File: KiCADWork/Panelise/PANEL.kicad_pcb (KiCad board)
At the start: 2 copper layers, 88.5 x 60.5 mm, 196 parts, among them J1 Screw_Terminal_01x01, J1 Screw_Terminal_01x02, J1 USB_C_Receptacle, J2 Screw_Terminal_01x01, J2 Screw_Terminal_01x02, J3 USB_C_Receptacle, J4 Conn_01x10_Socket, P1 USB_C_Plug, P2 USB_C_Plug, SW1 TK-6580B-1, SW2 SW_DIP_x01, U1 MCP73831T-2ACI/OT, U1 USB2422T-I/MJ, U2 TPS61023DRLR, U2 XB6096I2SV, U3 AMS1117-3.3, U3 NRF52833-QDAA-R7, U4 BQ24073RGT, U5 SIP32509DT-T1-GE3, U6 SIP32509DT-T1-GE3, Y1 X322524MOB4SI, Y1 XL7EL89CKI-111YLC-32M, Y2 X161032768KLD2SI

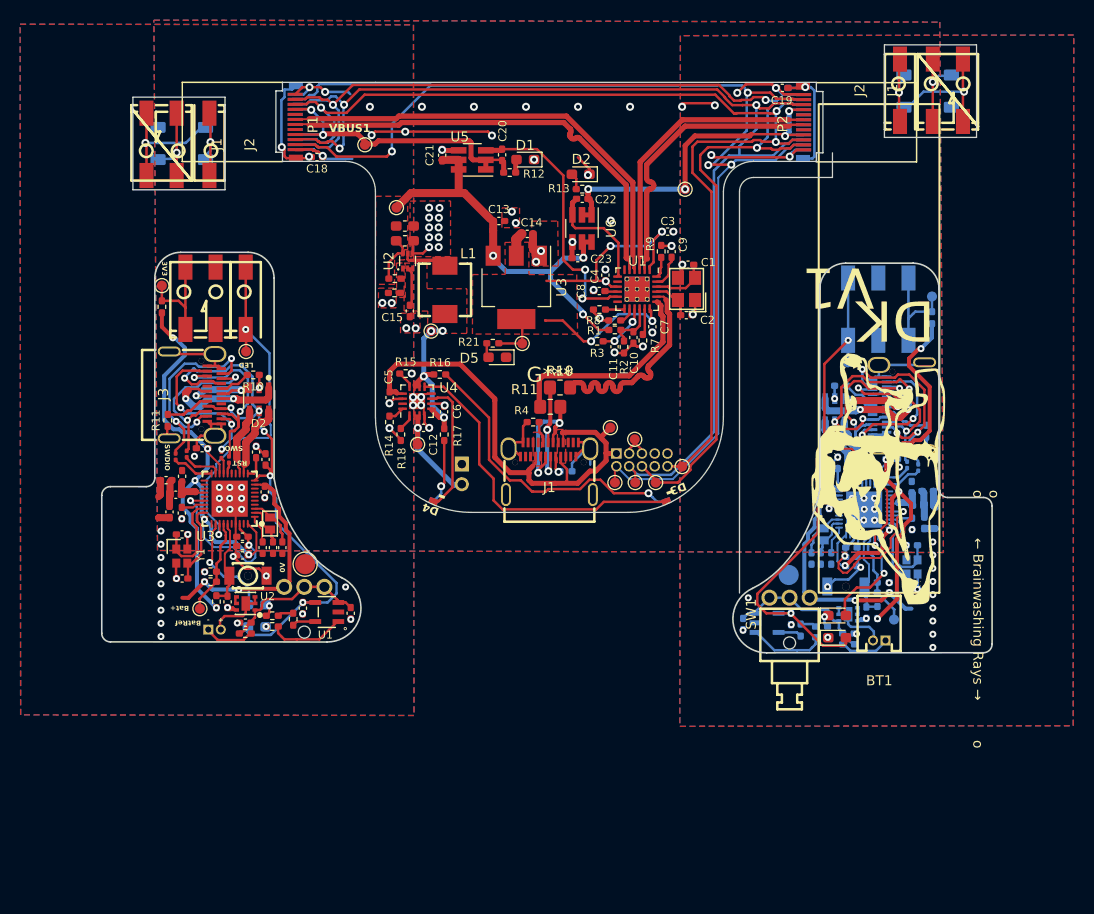
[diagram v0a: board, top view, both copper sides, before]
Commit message: Started mirror earrings and case
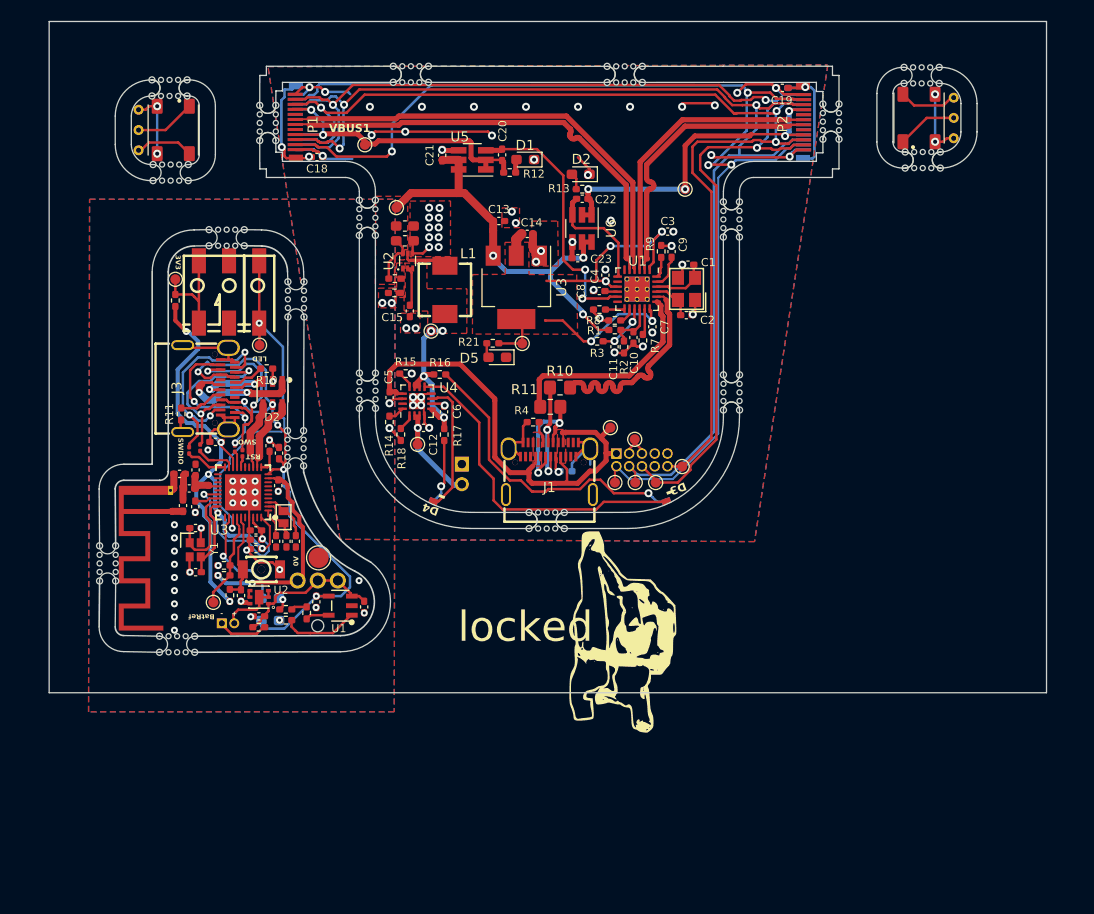
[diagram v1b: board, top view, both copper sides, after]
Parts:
- removed A, B, C, D, E: Board, kikit:Board
- removed the BT1 at (178.3, 114.7)
- removed the BT1 at (112.2, 113.6)
- removed the C1 at (115.0, 106.2)
- removed the C1 at (175.6, 107.3)
- removed the C10 at (117.3, 96.7)
- removed the C10 at (173.3, 97.8)
- removed the C11 at (109.0, 102.0)
- removed the C11 at (181.6, 103.1)
- removed the C12 at (117.2, 99.9)
- removed the C12 at (173.3, 101.0)
- removed the C13 at (125.8, 112.0)
- removed the C13 at (164.8, 113.1)
- removed the C14 at (113.5, 110.9)
- removed the C14 at (177.0, 111.9)
- removed the C15 at (119.0, 105.5)
- removed the C15 at (171.6, 106.6)
- removed the C16 at (118.0, 105.5)
- removed the C16 at (172.5, 106.6)
- removed the C17 at (115.0, 105.3)
- removed the C17 at (175.6, 106.4)
- removed the C18 at (115.3, 112.9)
- removed the C18 at (175.3, 114.0)
- removed the C19 at (121.0, 111.5)
- removed the C19 at (169.6, 112.6)
- removed the C2 at (117.0, 105.5)
- removed the C2 at (173.6, 106.6)
- removed the C3 at (109.0, 104.2)
- removed the C3 at (181.6, 105.2)
- removed the C4 at (109.0, 108.5)
- removed the C4 at (181.6, 109.6)
- removed the C5 at (107.4, 98.8)
- removed the C5 at (183.2, 99.8)
- removed the C6 at (111.0, 95.6)
- removed the C6 at (179.6, 96.7)
- removed the C7 at (115.0, 104.4)
- removed the C7 at (175.6, 105.5)
- removed the C8 at (109.0, 98.4)
- removed the C8 at (181.6, 99.5)
- removed the C9 at (116.4, 96.0)
- removed the C9 at (174.2, 97.0)
- removed the D1 at (174.1, 114.4)
- removed the D1 at (109.0, 65.3)
- removed the D1 at (183.2, 60.1)
- removed the D1 at (116.4, 113.4)
- removed the D2 at (116.7, 90.7)
- removed the D2 at (173.9, 91.8)
- removed the D4 at (174.1, 112.2)
- removed the D4 at (116.4, 111.2)
- removed the G*** at (178.4, 98.8)
- removed the G*** at (112.1, 97.8)
- removed the J1 at (116.8, 80.7)
- removed the J1 at (107.0, 65.4)
- removed the J1 at (185.2, 60.0)
- removed the J1 at (173.7, 81.8)
- removed the J2 at (110.8, 80.7)
- removed the J2 at (181.9, 60.0)
- removed the J2 at (110.2, 65.4)
- removed the J2 at (179.7, 81.8)
- removed the J3 at (110.3, 90.3)
- removed the J3 at (180.3, 91.4)
- removed the L1 at (108.4, 100.2)
- removed the L1 at (182.2, 101.3)
- removed the L2 at (107.8, 101.9)
- removed the L2 at (182.8, 103.0)
- removed the R1 at (118.0, 113.3)
- removed the R1 at (172.6, 114.4)
- removed the R10 at (116.1, 88.3)
- removed the R10 at (174.5, 89.4)
- removed the R11 at (107.6, 92.8)
- removed the R11 at (183.0, 93.9)
- removed the R12 at (118.0, 112.2)
- removed the R12 at (172.6, 113.3)
- removed the R13 at (111.8, 108.9)
- removed the R13 at (178.7, 109.9)
- removed the R14 at (111.8, 107.9)
- removed the R14 at (178.7, 108.9)
- removed the R2 at (112.4, 110.8)
- removed the R2 at (178.2, 111.9)
- removed the R3 at (115.3, 114.0)
- removed the R3 at (175.3, 115.1)
- removed the R4 at (120.0, 112.6)
- removed the R4 at (170.5, 113.7)
- removed the R5 at (113.7, 96.7)
- removed the R5 at (176.9, 97.8)
- removed the R6 at (112.9, 96.3)
- removed the R6 at (177.7, 97.3)
- removed the R7 at (108.4, 96.4)
- removed the R7 at (182.2, 97.5)
- removed the R8 at (109.5, 96.2)
- removed the R8 at (181.1, 97.2)
- removed the R9 at (107.0, 81.5)
- removed the R9 at (183.6, 82.6)
- removed the SW1 at (169.4, 110.5)
- removed the SW1 at (121.2, 109.4)
- removed the SW2 at (115.5, 108.3)
- removed the SW2 at (175.0, 109.3)
- removed the TP10 at (115.4, 86.0)
- removed the TP10 at (175.2, 87.0)
- removed the TP11 at (107.0, 79.4)
- removed the TP11 at (183.6, 80.5)
- removed the TP16 at (121.2, 107.1)
- removed the TP16 at (169.3, 108.2)
- removed the TP9 at (110.8, 111.5)
- removed the TP9 at (179.8, 112.6)
- removed the U1 at (123.4, 111.9)
- removed the U1 at (167.2, 113.0)
- removed the U2 at (115.3, 111.0)
- removed the U2 at (175.2, 112.1)
- removed the U3 at (113.7, 100.6)
- removed the U3 at (176.8, 101.7)
- removed the Y1 at (109.0, 106.3)
- removed the Y1 at (181.6, 107.4)
- removed the Y2 at (117.8, 103.1)
- removed the Y2 at (172.8, 104.2)
- added ANT1: ~, RF_Antenna:Texas_SWRA117D_2.4GHz_Left, F.Cu at (107.8, 101.9)
- added BT1: Battery, easyeda2kicad:CONN-TH_530480210, B.Cu at (113.6, 113.0)
- added C1: 1u, Capacitor_SMD:C_0402_1005Metric_Pad0.74x0.62mm_HandSolder, F.Cu at (116.3, 105.6)
- added C10: 4.7u, Capacitor_SMD:C_0402_1005Metric_Pad0.74x0.62mm_HandSolder, F.Cu at (118.6, 96.1)
- added C11: 100p, Capacitor_SMD:C_0402_1005Metric_Pad0.74x0.62mm_HandSolder, F.Cu at (110.3, 101.4)
- added C12: 4.7u, Capacitor_SMD:C_0402_1005Metric_Pad0.74x0.62mm_HandSolder, F.Cu at (118.6, 99.3)
- added C13: 10u, Capacitor_SMD:C_0402_1005Metric_Pad0.74x0.62mm_HandSolder, F.Cu at (127.1, 111.4)
- added C14: 100n, Capacitor_SMD:C_0402_1005Metric_Pad0.74x0.62mm_HandSolder, F.Cu at (114.9, 110.2)
- added C15: 8p, Capacitor_SMD:C_0402_1005Metric_Pad0.74x0.62mm_HandSolder, F.Cu at (120.3, 104.9)
- added C16: 8p, Capacitor_SMD:C_0402_1005Metric_Pad0.74x0.62mm_HandSolder, F.Cu at (119.4, 104.9)
- added C17: NC, Capacitor_SMD:C_0402_1005Metric_Pad0.74x0.62mm_HandSolder, F.Cu at (116.3, 104.7)
- added C18: 100n, Capacitor_SMD:C_0402_1005Metric_Pad0.74x0.62mm_HandSolder, F.Cu at (116.6, 112.3)
- added C19: 10u, Capacitor_SMD:C_0402_1005Metric_Pad0.74x0.62mm_HandSolder, F.Cu at (122.3, 110.9)
- added C2: 100n, Capacitor_SMD:C_0402_1005Metric_Pad0.74x0.62mm_HandSolder, F.Cu at (118.3, 104.9)
- added C3: 12p, Capacitor_SMD:C_0402_1005Metric_Pad0.74x0.62mm_HandSolder, F.Cu at (110.3, 103.5)
- added C4: 12p, Capacitor_SMD:C_0402_1005Metric_Pad0.74x0.62mm_HandSolder, F.Cu at (110.3, 107.9)
- added C5: 1.2p, Capacitor_SMD:C_0402_1005Metric_Pad0.74x0.62mm_HandSolder, F.Cu at (108.7, 98.1)
- added C6: 100n, Capacitor_SMD:C_0402_1005Metric_Pad0.74x0.62mm_HandSolder, F.Cu at (112.3, 95.0)
- added C7: 1u, Capacitor_SMD:C_0402_1005Metric_Pad0.74x0.62mm_HandSolder, F.Cu at (116.3, 103.8)
- added C8: 1p, Capacitor_SMD:C_0402_1005Metric_Pad0.74x0.62mm_HandSolder, F.Cu at (110.3, 97.8)
- added C9: 4.7u, Capacitor_SMD:C_0402_1005Metric_Pad0.74x0.62mm_HandSolder, F.Cu at (117.7, 95.3)
- added D1: 2758, easyeda2kicad:SOL320P540X170-4N, F.Cu at (108.1, 63.9)
- added D1: 2758, easyeda2kicad:SOL320P540X170-4N, F.Cu at (182.3, 62.8)
- added D1: RED LED, LED_SMD:LED_0603_1608Metric_Pad1.05x0.95mm_HandSolder, B.Cu at (117.8, 112.7)
- added D2: USBLC6-2SC6_C2687116, easyeda2kicad:SOT-23-6_L2.9-W1.6-P0.95-LS2.8-BL, F.Cu at (118.0, 90.1)
- added D4: BLUE LED, LED_SMD:LED_0603_1608Metric_Pad1.05x0.95mm_HandSolder, B.Cu at (117.8, 110.5)
- added G***: LOGO, CustomPads:OT1, F.Cu at (152.7, 113.7)
- added G***: LOGO, CustomPads:OT2, B.Cu at (113.5, 97.1)
- added J1: Screw_Terminal_01x01, easyeda2kicad:CONN-SMD_custom1, F.Cu at (118.2, 80.1)
- added J2: Screw_Terminal_01x02, easyeda2kicad:CONN-SMD_2059-302, F.Cu at (112.2, 80.1)
- added J3: USB_C_Receptacle, easyeda2kicad:TYPE-C-SMD_C9900025773, F.Cu at (111.6, 89.7)
- added L1: 4.7n, Inductor_SMD:L_0402_1005Metric_Pad0.77x0.64mm_HandSolder, F.Cu at (109.7, 99.6)
- added L2: 2.2n, Inductor_SMD:L_0402_1005Metric_Pad0.77x0.64mm_HandSolder, F.Cu at (109.1, 101.3)
- added R1: 2k, Resistor_SMD:R_0402_1005Metric_Pad0.72x0.64mm_HandSolder, F.Cu at (119.3, 112.7)
- added R10: 5k1, Resistor_SMD:R_0402_1005Metric_Pad0.72x0.64mm_HandSolder, F.Cu at (117.4, 87.7)
- added R11: 5k1, Resistor_SMD:R_0402_1005Metric_Pad0.72x0.64mm_HandSolder, F.Cu at (108.9, 92.2)
- added R12: 220, Resistor_SMD:R_0402_1005Metric_Pad0.72x0.64mm_HandSolder, F.Cu at (119.3, 111.6)
- added R13: 100k, Resistor_SMD:R_0402_1005Metric_Pad0.72x0.64mm_HandSolder, F.Cu at (113.2, 108.2)
- added R14: 33k, Resistor_SMD:R_0402_1005Metric_Pad0.72x0.64mm_HandSolder, F.Cu at (113.2, 107.2)
- added R2: 2k, Resistor_SMD:R_0402_1005Metric_Pad0.72x0.64mm_HandSolder, F.Cu at (113.7, 110.2)
- added R3: 100, Resistor_SMD:R_0402_1005Metric_Pad0.72x0.64mm_HandSolder, F.Cu at (116.6, 113.4)
- added R4: 4k99, Resistor_SMD:R_0402_1005Metric_Pad0.72x0.64mm_HandSolder, F.Cu at (121.4, 112.0)
- added R5: NF, Resistor_SMD:R_0201_0603Metric, F.Cu at (115.0, 96.1)
- added R6: NF, Resistor_SMD:R_0201_0603Metric, F.Cu at (114.2, 95.6)
- added R7: NF, Resistor_SMD:R_0201_0603Metric, F.Cu at (109.7, 95.8)
- added R8: NF, Resistor_SMD:R_0201_0603Metric, F.Cu at (110.8, 95.5)
- added R9: 470, Resistor_SMD:R_0402_1005Metric_Pad0.72x0.64mm_HandSolder, F.Cu at (108.3, 80.9)
- added REF**: mouse-bit-1.6mm-slot, Panelization:mouse-bit-1.6mm-slot, F.Cu at (163.6, 90.0)
- added REF**: mouse-bit-1.6mm-slot, Panelization:mouse-bit-1.6mm-slot, F.Cu at (163.6, 72.8)
- added REF**: mouse-bit-1.6mm-slot, Panelization:mouse-bit-1.6mm-slot, F.Cu at (107.8, 59.8)
- added REF**: mouse-bit-1.6mm-slot, Panelization:mouse-bit-1.6mm-slot, B.Cu at (113.4, 74.7)
- added REF**: mouse-bit-1.6mm-slot, Panelization:mouse-bit-1.6mm-slot, B.Cu at (107.9, 68.2)
- added REF**: mouse-bit-1.6mm-slot, Panelization:mouse-bit-1.6mm-slot, B.Cu at (120.3, 95.6)
- added REF**: mouse-bit-1.6mm-slot, Panelization:mouse-bit-1.6mm-slot, B.Cu at (182.6, 58.5)
- added REF**: mouse-bit-1.6mm-slot, Panelization:mouse-bit-1.6mm-slot, B.Cu at (120.3, 80.8)
- added REF**: mouse-bit-1.6mm-slot, Panelization:mouse-bit-1.6mm-slot, B.Cu at (108.5, 115.1)
- added REF**: mouse-bit-1.6mm-slot, Panelization:mouse-bit-1.6mm-slot, B.Cu at (101.6, 107.0)
- added REF**: mouse-bit-1.6mm-slot, Panelization:mouse-bit-1.6mm-slot, F.Cu at (145.3, 102.8)
- added REF**: mouse-bit-1.6mm-slot, Panelization:mouse-bit-1.6mm-slot, F.Cu at (127.4, 89.9)
- added REF**: mouse-bit-1.6mm-slot, Panelization:mouse-bit-1.6mm-slot, F.Cu at (117.5, 63.2)
- added REF**: mouse-bit-1.6mm-slot, Panelization:mouse-bit-1.6mm-slot, F.Cu at (127.4, 72.7)
- added REF**: mouse-bit-1.6mm-slot, Panelization:mouse-bit-1.6mm-slot, F.Cu at (131.8, 58.4)
- added REF**: mouse-bit-1.6mm-slot, Panelization:mouse-bit-1.6mm-slot, F.Cu at (173.5, 63.1)
- added REF**: mouse-bit-1.6mm-slot, Panelization:mouse-bit-1.6mm-slot, F.Cu at (182.7, 66.9)
- added REF**: mouse-bit-1.6mm-slot, Panelization:mouse-bit-1.6mm-slot, F.Cu at (153.0, 58.4)
- added SW1: TK-6580B-1, easyeda2kicad:SW-TH_TK-6580B-1, B.Cu at (122.5, 108.7)
- added SW2: SW_DIP_x01, easyeda2kicad:KEY-SMD_L3.0-W2.5-LS4.0, F.Cu at (116.9, 107.6)
- added TP1: TestPoint, TestPoint:TestPoint_THTPad_D1.0mm_Drill0.5mm, B.Cu at (104.7, 66.0)
- added TP1: TestPoint, TestPoint:TestPoint_THTPad_D1.0mm_Drill0.5mm, B.Cu at (185.7, 60.7)
- added TP10: TestPoint, TestPoint:TestPoint_Pad_D1.0mm, F.Cu at (116.7, 85.3)
- added TP11: TestPoint, TestPoint:TestPoint_Pad_D1.0mm, F.Cu at (108.3, 78.8)
- added TP16: TestPoint, TestPoint:TestPoint_Pad_D2.0mm, F.Cu at (122.6, 106.5)
- added TP2: TestPoint, TestPoint:TestPoint_THTPad_D1.0mm_Drill0.5mm, B.Cu at (185.7, 62.7)
- added TP2: TestPoint, TestPoint:TestPoint_THTPad_D1.0mm_Drill0.5mm, B.Cu at (104.7, 63.9)
- added TP3: TestPoint, TestPoint:TestPoint_THTPad_D1.0mm_Drill0.5mm, B.Cu at (185.7, 64.8)
- added TP3: TestPoint, TestPoint:TestPoint_THTPad_D1.0mm_Drill0.5mm, B.Cu at (104.7, 61.9)
- added TP9: TestPoint, TestPoint:TestPoint_Pad_D1.0mm, F.Cu at (112.1, 110.9)
- added U1: MCP73831T-2ACI/OT, easyeda2kicad:SOT-23-5_L3.0-W1.7-P0.95-LS2.8-BL, F.Cu at (124.7, 111.3)
- added U2: XB6096I2SV, easyeda2kicad:WDFN-6_L2.0-W2.0-P0.65-BL-EP, F.Cu at (116.7, 110.4)
- added U3: NRF52833-QDAA-R7, easyeda2kicad:QFN-40_L5.0-W5.0-P0.40-TL-EP3.6, F.Cu at (115.1, 100.0)
- added Y1: XL7EL89CKI-111YLC-32M, easyeda2kicad:CRYSTAL-SMD_4P-L2.0-W1.6-BL, F.Cu at (110.3, 105.7)
- added Y2: X161032768KLD2SI, easyeda2kicad:CRYSTAL-SMD_L1.6-W1.0, F.Cu at (119.1, 102.5)
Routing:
- net (no net): track 818.1 -> 418.6 mm, vias 61 -> 32
- net +3V3: track 151.6 -> 97.5 mm, vias 17 -> 11
- net GND: track 187.7 -> 141.1 mm, vias 127 -> 93
- net Net-(D4-K): track 16.2 -> 14.7 mm, vias 2 -> 1
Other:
- board size 88.5 x 60.5 mm -> 99.2 x 66.8 mm
- board text added: "locked"
- board text removed: "Bat+"
